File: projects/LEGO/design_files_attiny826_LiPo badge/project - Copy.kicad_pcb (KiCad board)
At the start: 2 copper layers, 86 x 54 mm, 80 parts, among them J1 USB-MICRO, J2 BAT, J3 UDPI, J4 Pin, Q1 SOT-23, Q2 SOT-323, Q3 SOT-223, SW1 SW_SPST, U1 ATtiny826, U10 SOIC-8, U2 MCP73833, U3 VQFN-20, U4 UFBGA-15, U5 QFN-20, U6 TSSOP-20, U7 SOT-23-5, U8 TDFN-8, U9 MSOP-8

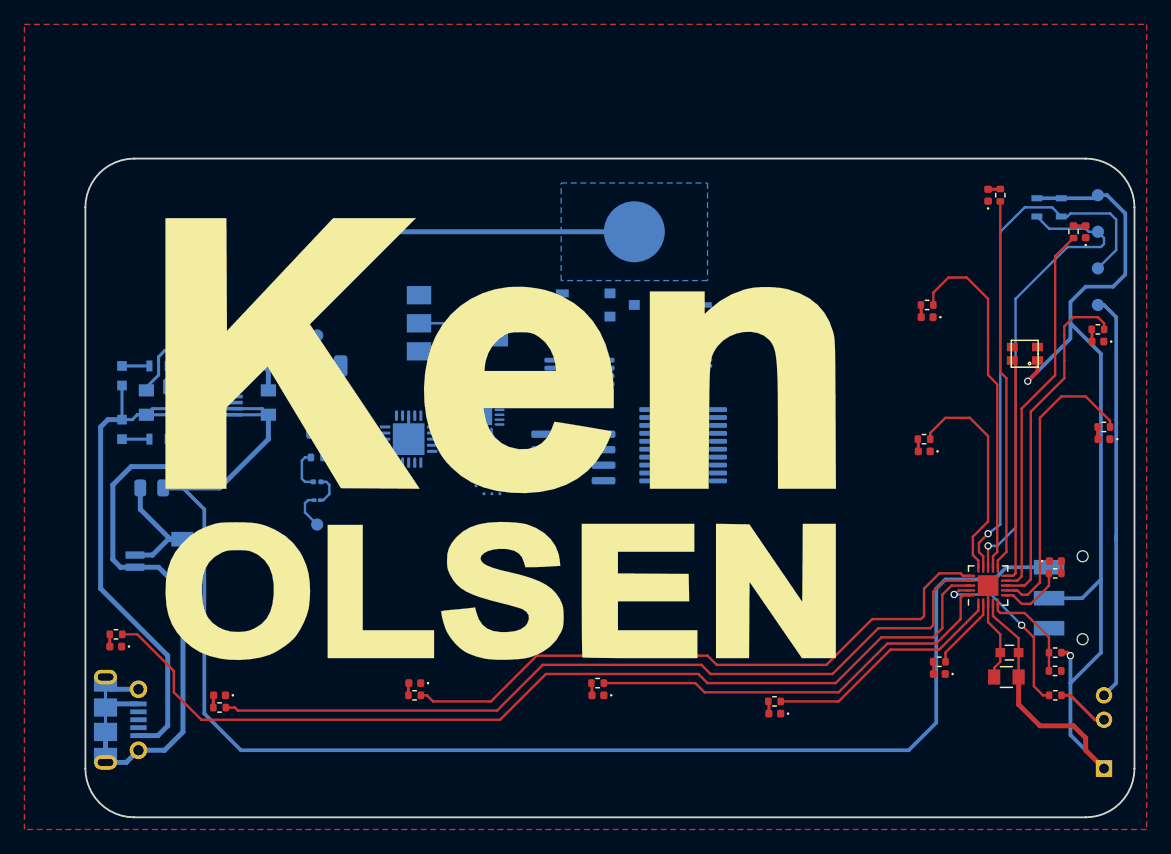
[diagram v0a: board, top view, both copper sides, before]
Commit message: Updaes
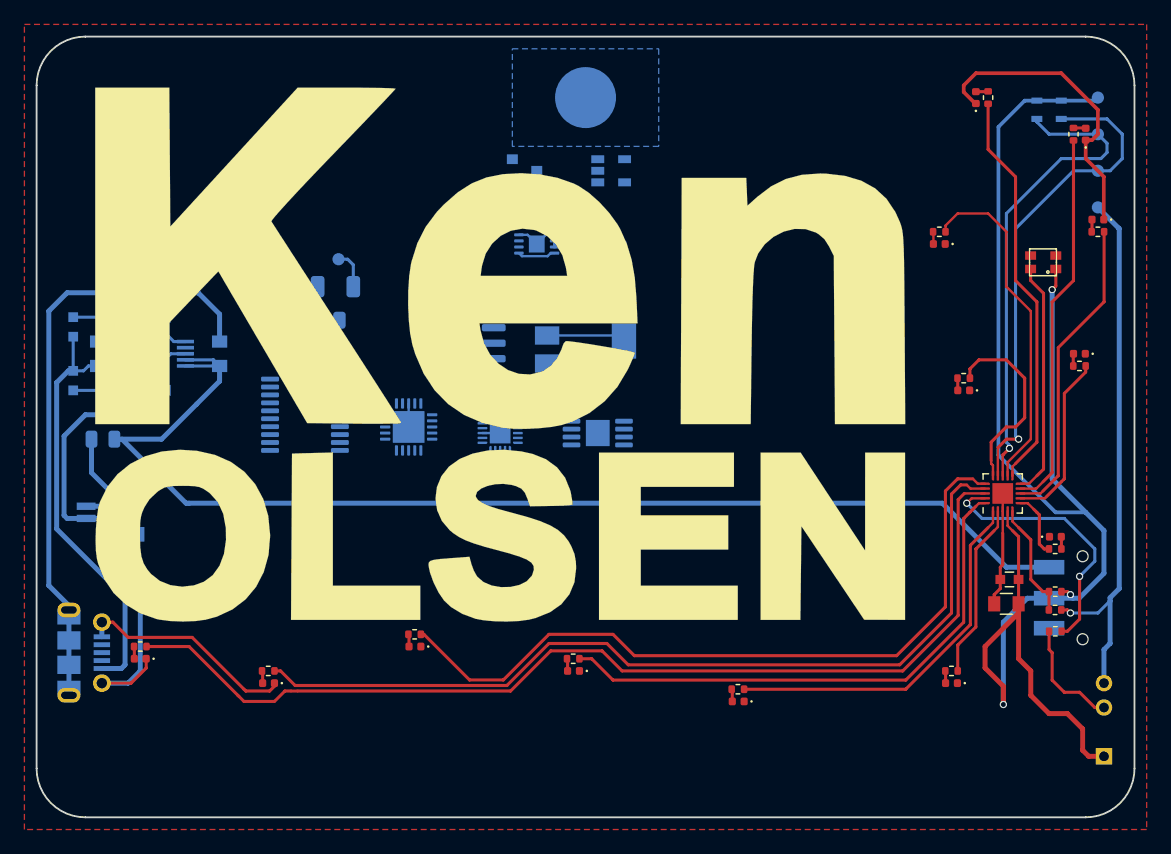
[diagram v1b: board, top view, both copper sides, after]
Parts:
- moved SYM7 69.3 mm to (115.0, 110.2)
- moved SYM6 43.1 mm to (127.3, 100.0)
- moved U6 31.1 mm to (125.3, 87.2)
- moved SYM5 23.0 mm to (160.3, 105.2)
- moved TP1 22.0 mm to (123.3, 74.5)
- moved U4 20.7 mm to (137.3, 72.2)
- moved R8 17.7 mm to (123.5, 76.7)
- moved U8 15.6 mm to (144.3, 73.2)
- moved R22 14.0 mm to (123.8, 79.0)
- moved Q1 13.6 mm to (143.3, 67.2)
- moved U10 13.5 mm to (138.3, 80.7)
- moved U7 12.1 mm to (150.4, 67.2)
- moved J4 11.7 mm to (148.3, 61.2)
- moved Q3 10.5 mm to (148.3, 80.7)
- moved R19 10.1 mm to (123.8, 81.0)
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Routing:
- net GND: track 157.9 -> 200.0 mm, vias 0 -> 1
- net VCC: track 95.1 -> 124.9 mm, vias 2 -> 3
- net +BATT: track 120.5 -> 98.0 mm
- net /D15: track 19.9 -> 30.8 mm
- net /D2: track 24.8 -> 14.2 mm
- net /D14: track 34.7 -> 45.0 mm
- net /D11: track 51.6 -> 61.8 mm
- net /D16: track 5.83 -> 14.5 mm
- net /UPDI: track 15.0 -> 22.0 mm
- net Net-(RL2-Pad1): track 3.70 -> 8.92 mm
- net /D12: track 67.8 -> 72.8 mm
- net Net-(J3-Pad3): track 4.31 -> 9.29 mm
- net /D13: track 80.2 -> 84.6 mm
- net /SCL: track 44.1 -> 40.3 mm
- net /D3: track 28.4 -> 25.3 mm
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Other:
- board size 86 x 54 mm -> 90 x 64 mm
- board text removed: "86 x 54"
